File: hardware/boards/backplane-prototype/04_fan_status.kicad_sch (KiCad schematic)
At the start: 14 parts, among them J11 12V 3-WIRE FAN, J12 DS18B20 EXT SUPPLY, J9 12V 3-WIRE FAN, Q1 AO3407A, Q2 2N7002, Q3 AO3407A, Q4 2N7002

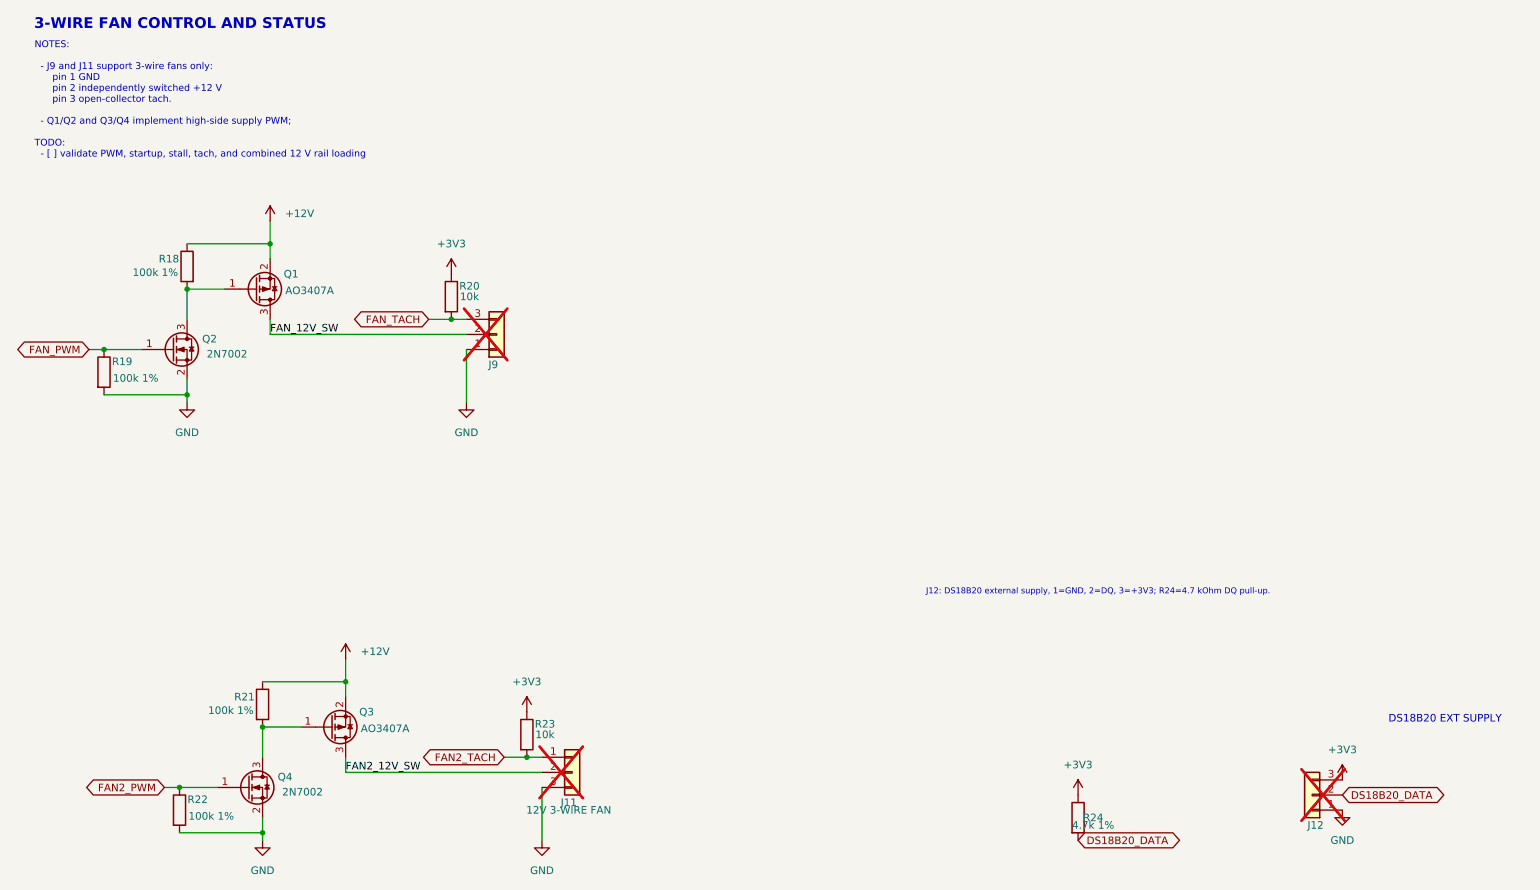
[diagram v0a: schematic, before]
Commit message: checkpoint: save fan and buck schematic edits
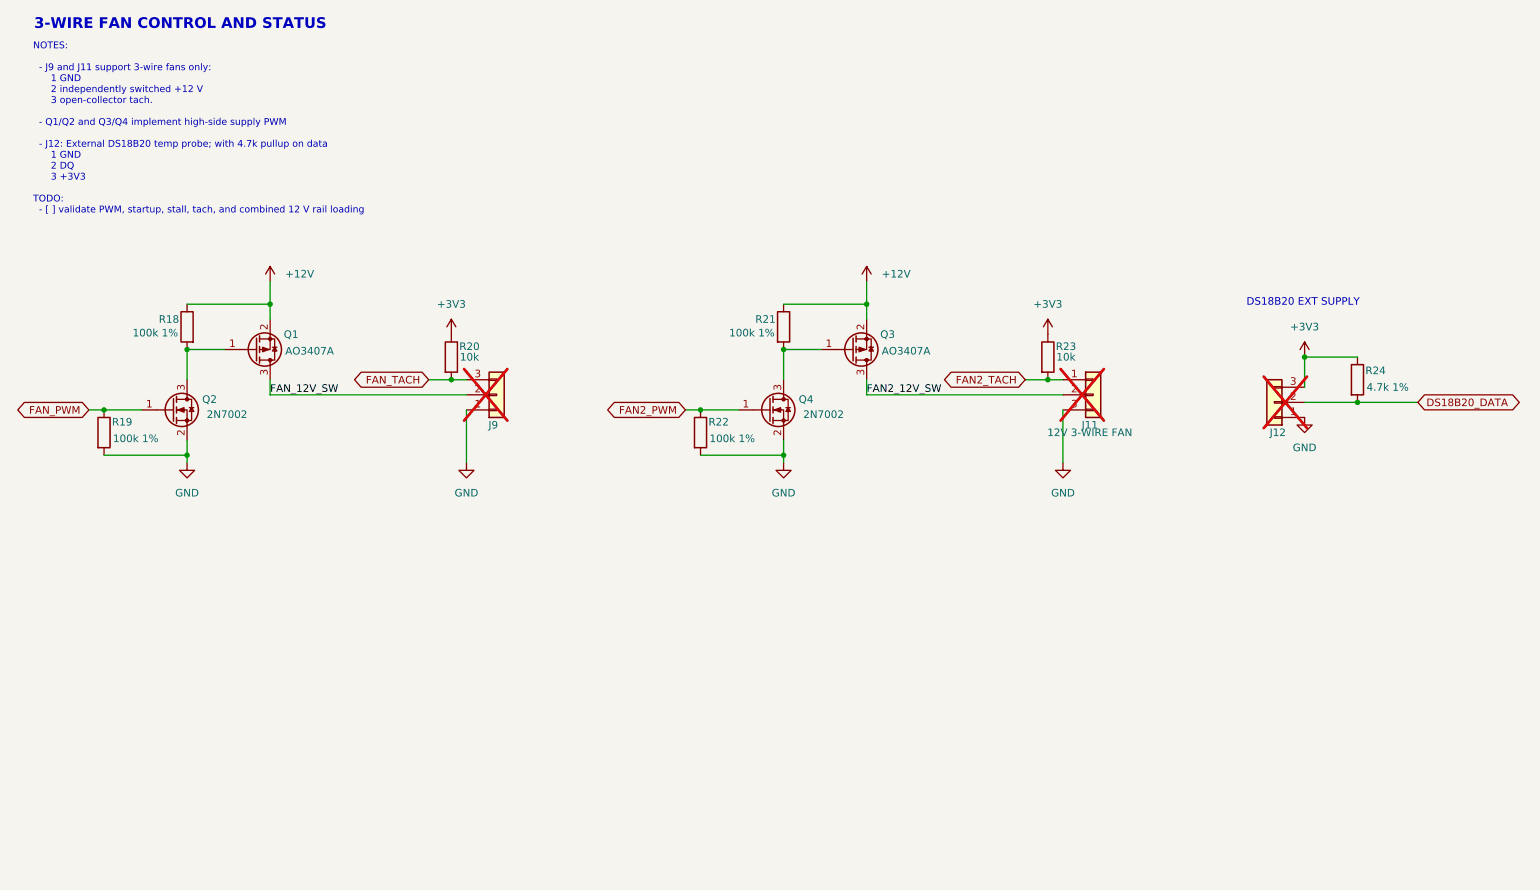
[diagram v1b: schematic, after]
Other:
- note added: "NOTES: - J9 and J11 support 3-wire fans only: 1 GND 2 independently switched +12 V 3 open-collector tach. - Q1/Q2 and Q3/Q4 implement high-side supply PWM - J12: External DS18B20 temp probe; with 4.7k pullup on data 1 GND 2 DQ 3 +3V3 TODO: - [ ] validate PWM, startup, stall, tach, and combined 12 V rail loading"
- note removed: "J12: DS18B20 external supply, 1=GND, 2=DQ, 3=+3V3; R24=4.7 kOhm DQ pull-up."
- note removed: "NOTES: - J9 and J11 support 3-wire fans only: pin 1 GND pin 2 independently switched +12 V pin 3 open-collector tach. - Q1/Q2 and Q3/Q4 implement high-side supply PWM; TODO: - [ ] validate PWM, startup, stall, tach, and combined 12 V rail loading"
- moved on the sheet: J11, J12, J9, Q1, Q2, Q3, Q4, R18, R19, R20, R21, R22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
